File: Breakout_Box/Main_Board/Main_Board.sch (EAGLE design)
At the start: 18 parts, among them CN1 19PIN_LEMO

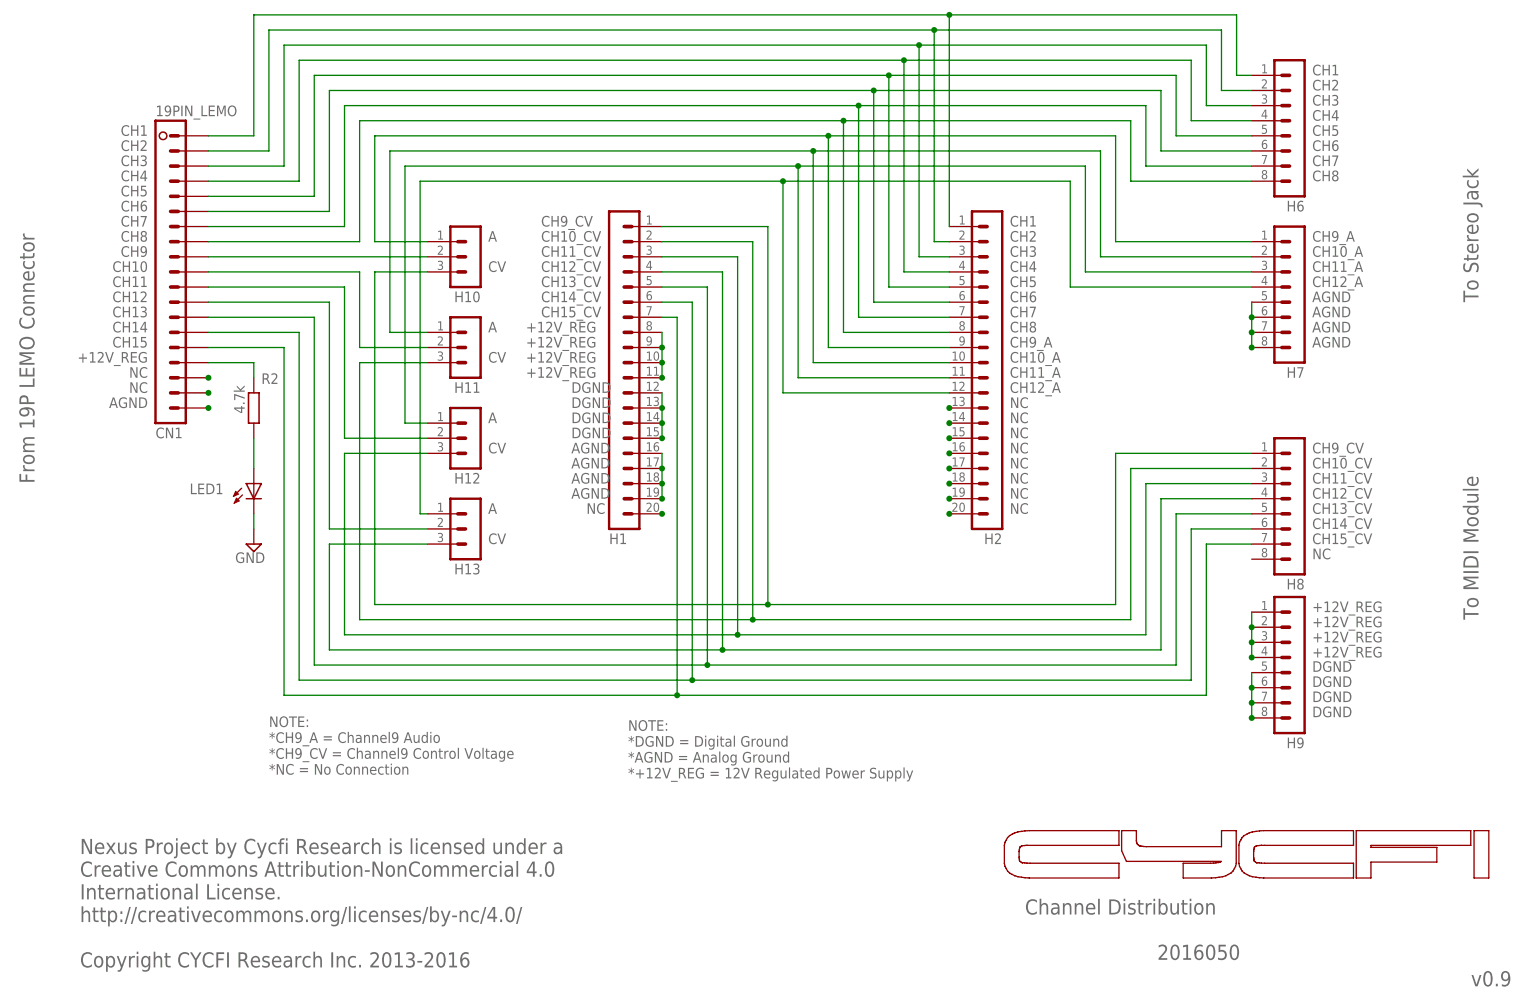
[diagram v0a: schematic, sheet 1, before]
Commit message: Licenses
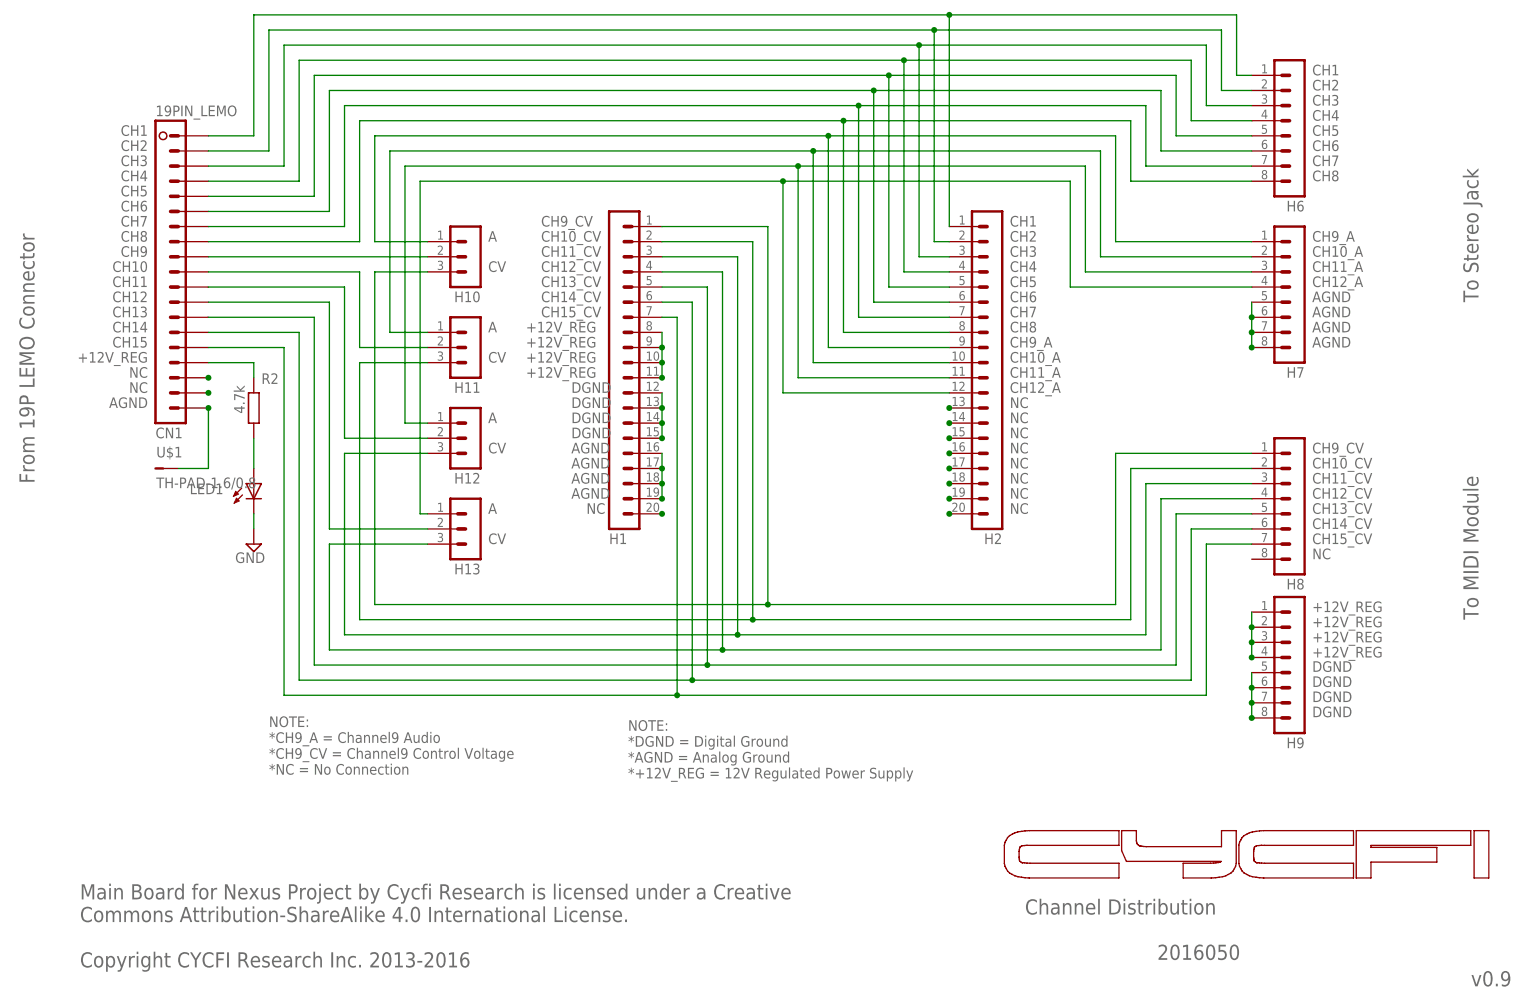
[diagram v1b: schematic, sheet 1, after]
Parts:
- added U$1: TH-PAD-1.6/0.8, CYCFI_Con:TH-PAD-1.6/0.8
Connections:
- net AGND: now also U$1.P
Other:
- note added: "MIDI Module for Nexus Project by Cycfi Research is licensed under a Creative Commons Attribution-ShareAlike 4.0 International License. Copyright CYCFI Research Inc. 2013-2016"
- note added: "Main Board for Nexus Project by Cycfi Research is licensed under a Creative Commons Attribution-ShareAlike 4.0 International License. Copyright CYCFI Research Inc. 2013-2016"
- note removed: "Nexus Project by Cycfi Research is licensed under a Creative Commons Attribution-NonCommercial 4.0 International License. http://creativecommons.org/licenses/by-nc/4.0/ Copyright CYCFI Research Inc. 2013-2016"
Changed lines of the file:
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@@
 <part name="CN1" library="CYCFI_Con" deviceset="19PIN_LEMO" device=""/>
 <part name="D1" library="CYCFI_diode" deviceset="FM4007W" device=""/>
+<part name="U$1" library="CYCFI_Con" deviceset="TH-PAD-1.6/0.8" device=""/>
 </parts>
 <sheets>
@@
 <text x="175.26" y="86.36" size="1.778" layer="95">NC</text>
 <text x="104.14" y="86.36" size="1.778" layer="95">NC</text>
-<text x="19.05" y="10.16" size="2.54" layer="95">Nexus Project by Cycfi Research is licensed under a
-Creative Commons Attribution-NonCommercial 4.0
-International License.
-http://creativecommons.org/licenses/by-nc/4.0/
+<text x="19.05" y="10.16" size="2.54" layer="95">Main Board for Nexus Project by Cycfi Research is licensed under a Creative
+Commons Attribution-ShareAlike 4.0 International License.
 Copyright CYCFI Research Inc. 2013-2016</text>
 <text x="30.48" y="149.86" size="1.778" layer="95" rot="MR0">CH1</text>
@@
 <instance part="H13" gate="G$1" x="85.09" y="83.82" rot="R180"/>
 <instance part="CN1" gate="G$1" x="33.02" y="125.73" rot="MR180"/>
+<instance part="U$1" gate="G$1" x="33.02" y="93.98"/>
 </instances>
 <busses>
@@
 <junction x="40.64" y="104.14"/>
 <label x="30.48" y="104.14" size="1.778" layer="95" rot="MR0"/>
+<wire x1="40.64" y1="104.14" x2="40.64" y2="93.98" width="0.1524" layer="91"/>
+<pinref part="U$1" gate="G$1" pin="P"/>
+<wire x1="40.64" y1="93.98" x2="35.56" y2="93.98" width="0.1524" layer="91"/>
 </segment>
 </net>
@@
 <text x="80.01" y="125.095" size="1.778" layer="95">+12V IN</text>
 <text x="86.36" y="122.555" size="1.778" layer="95">GND</text>
-<text x="12.7" y="12.7" size="2.54" layer="95">Nexus Project by Cycfi Research is licensed under a
-Creative Commons Attribution-NonCommercial 4.0
-International License.
-http://creativecommons.org/licenses/by-nc/4.0/
+<text x="12.7" y="12.7" size="2.54" layer="95">MIDI Module for Nexus Project by Cycfi Research is licensed under a
+Creative Commons Attribution-ShareAlike 4.0 International License.
 Copyright CYCFI Research Inc. 2013-2016</text>
 <text x="200.025" y="11.43" size="2.54" layer="95">2016050</text>

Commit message: *Edit Logo *Check BOM *Added 19P Connector Files
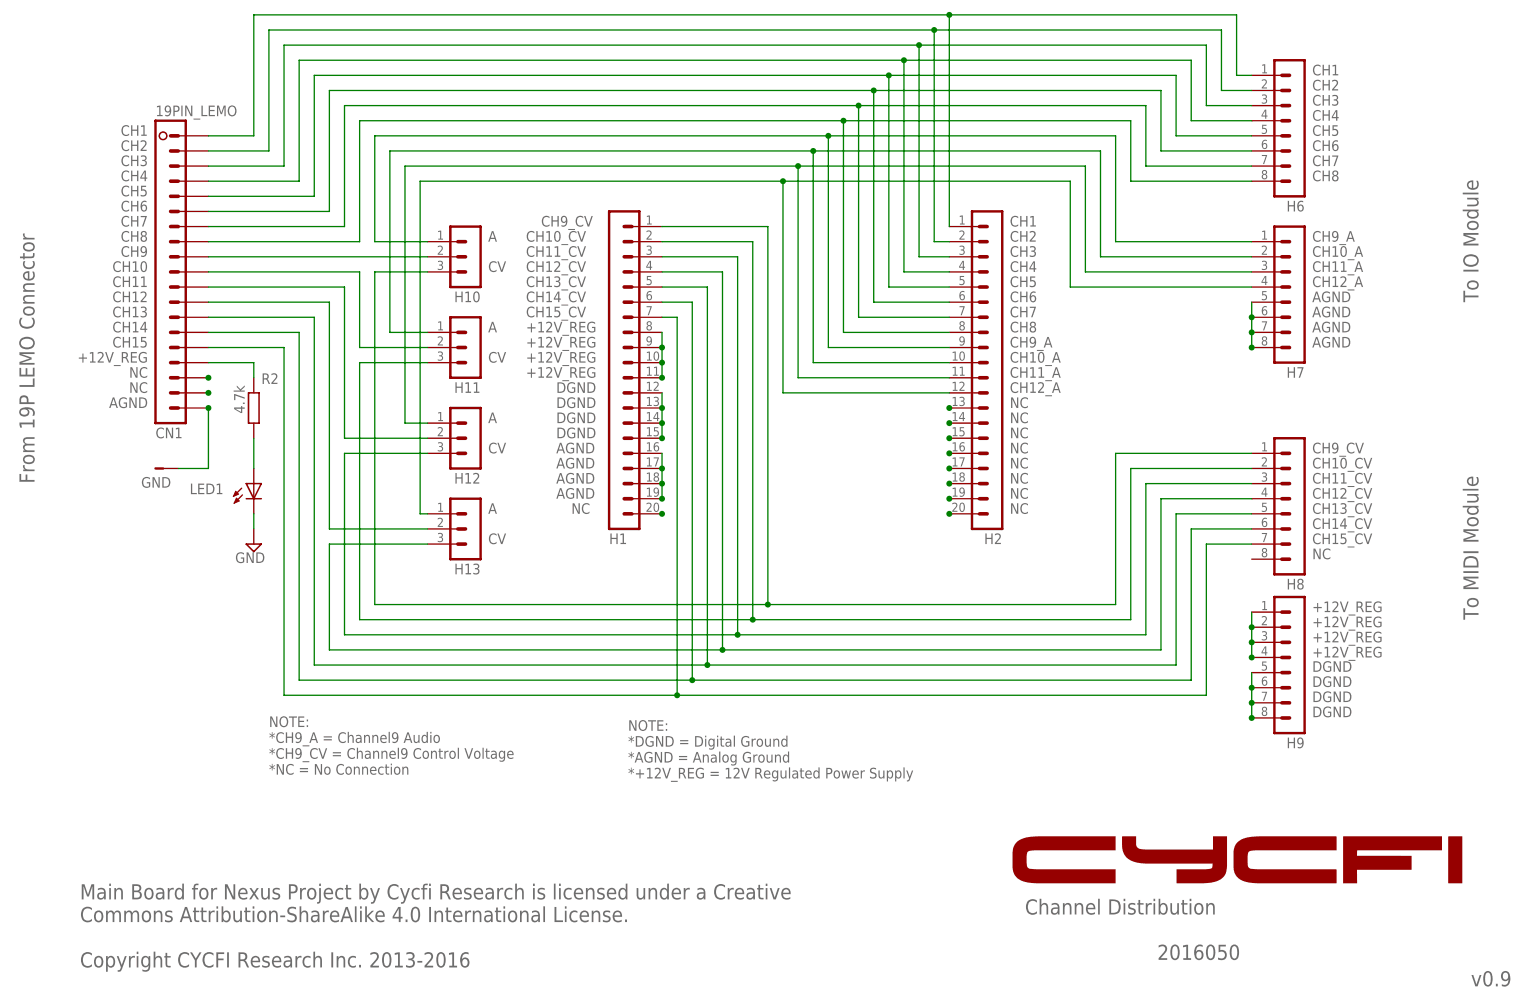
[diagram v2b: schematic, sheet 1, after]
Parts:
- renumbered U$1 to GND
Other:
- note added: "To IO Module"
- note removed: "MIDI Module for Nexus Project by Cycfi Research is licensed under a Creative Commons Attribution-ShareAlike 4.0 International License. Copyright CYCFI Research Inc. 2013-2016"
- note removed: "To Stereo Jack"
